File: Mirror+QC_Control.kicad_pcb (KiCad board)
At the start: 2 copper layers, 48.5 x 84 mm, 29 parts, among them J1 3220-10-0300-00, J2 Screw_Terminal_01x04, J3 Screw_Terminal_01x06, U1 LT1012, U10 LT1012, U11 LT1012, U2 LM4040DBZ-2.0, U3 LT1012, U4 LM4040DBZ-2.0, U5 LT1012, U6 LT1012, U7 Teensy4.0

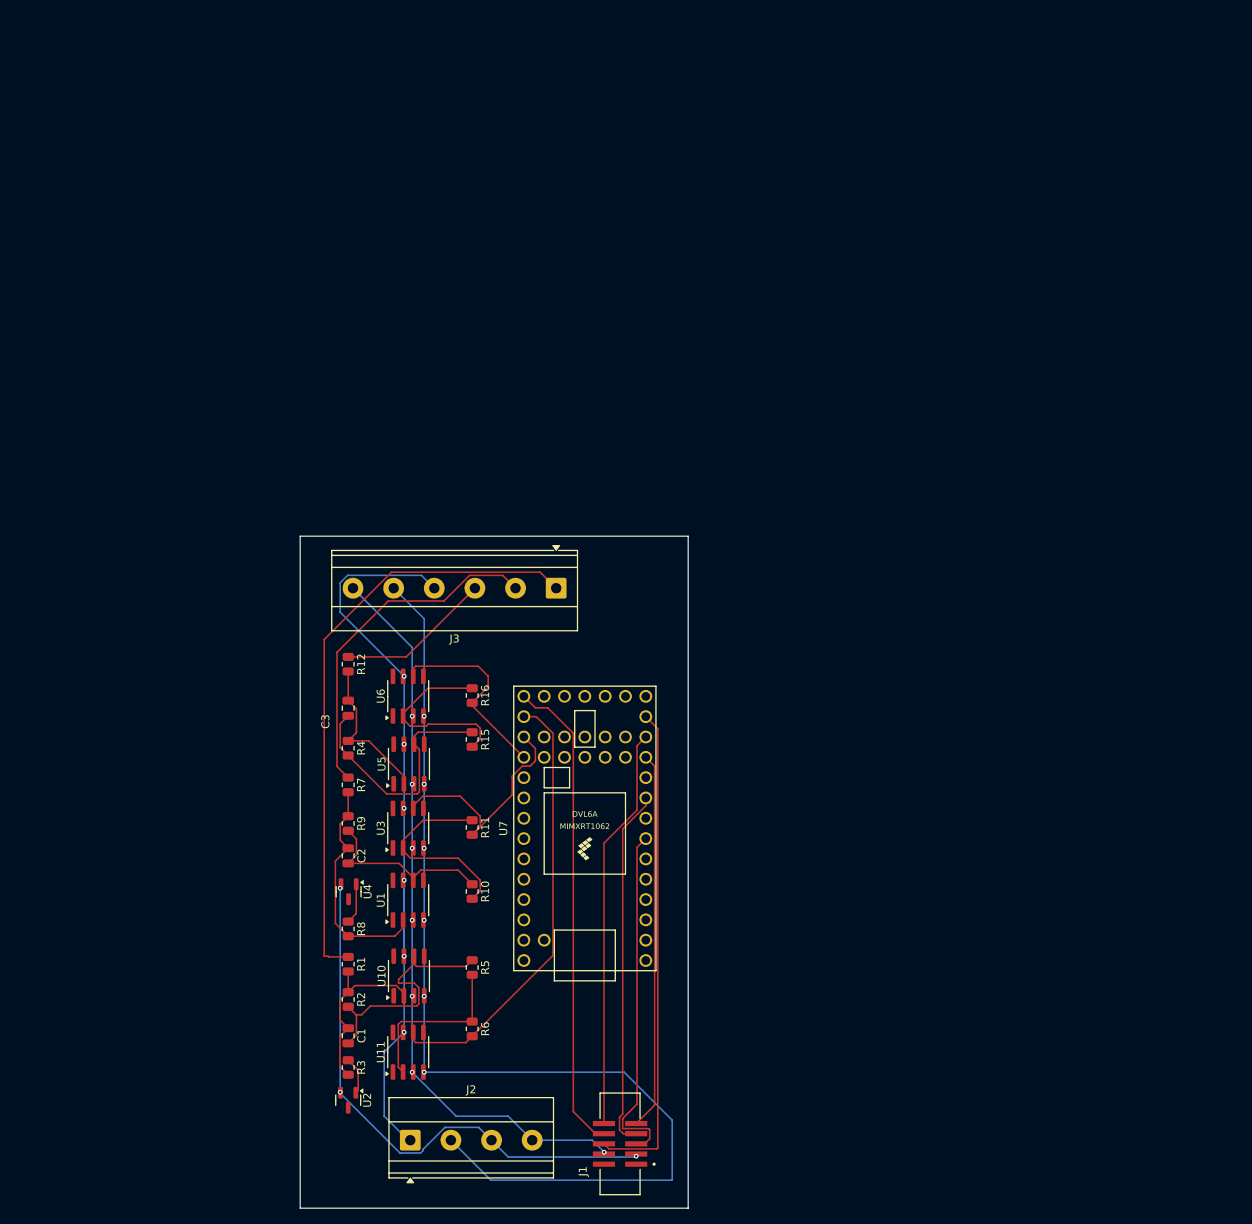
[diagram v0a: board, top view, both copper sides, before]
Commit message: changes after DR1
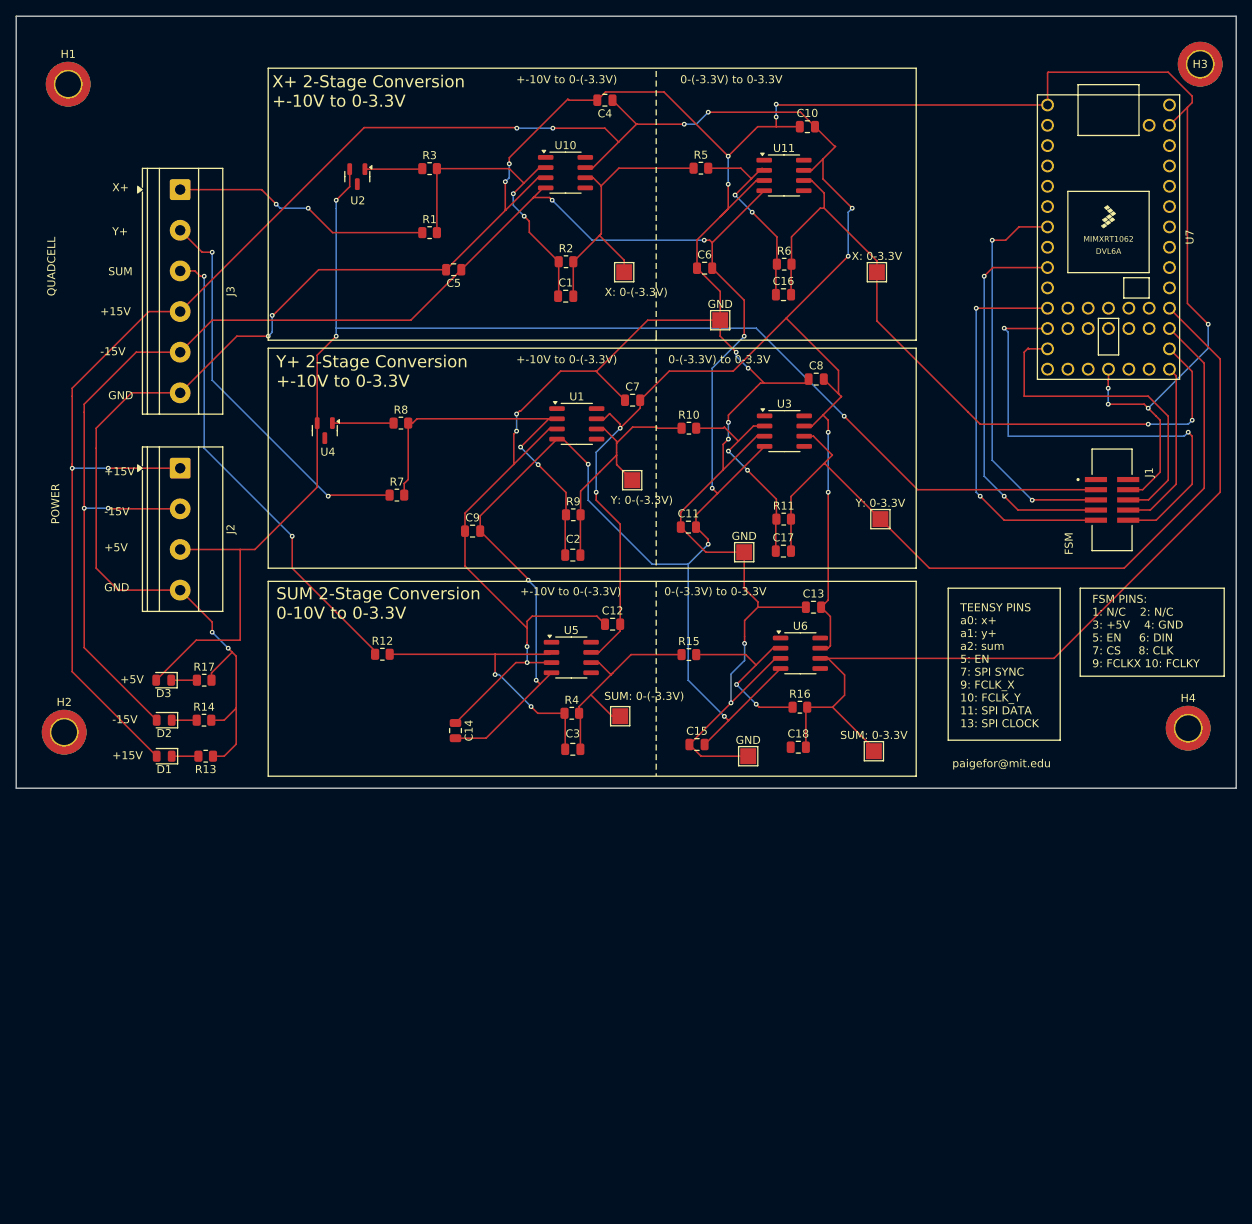
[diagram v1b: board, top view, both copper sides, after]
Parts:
- added C10: 0.1muF, Capacitor_SMD:C_0805_2012Metric, F.Cu at (118.4, 38.3)
- added C11: 0.1muF, Capacitor_SMD:C_0805_2012Metric, F.Cu at (103.5, 88.4)
- added C12: 0.1muF, Capacitor_SMD:C_0805_2012Metric, F.Cu at (94.0, 100.5)
- added C13: 0.1muF, Capacitor_SMD:C_0805_2012Metric, F.Cu at (119.2, 98.4)
- added C14: 0.1muF, Capacitor_SMD:C_0805_2012Metric, F.Cu at (74.4, 113.8)
- added C15: 0.1muF, Capacitor_SMD:C_0805_2012Metric, F.Cu at (104.6, 115.5)
- added C16: C, Capacitor_SMD:C_0805_2012Metric, F.Cu at (115.4, 59.3)
- added C17: C, Capacitor_SMD:C_0805_2012Metric, F.Cu at (115.4, 91.4)
- added C18: C, Capacitor_SMD:C_0805_2012Metric, F.Cu at (117.3, 115.9)
- added C4: 0.1muF, Capacitor_SMD:C_0805_2012Metric, F.Cu at (93.1, 35.0)
- added C5: 0.1muF, Capacitor_SMD:C_0805_2012Metric, F.Cu at (74.2, 56.2)
- added C6: 0.1muF, Capacitor_SMD:C_0805_2012Metric, F.Cu at (105.5, 56.0)
- added C7: 0.1muF, Capacitor_SMD:C_0805_2012Metric, F.Cu at (96.5, 72.5)
- added C8: 0.1muF, Capacitor_SMD:C_0805_2012Metric, F.Cu at (119.5, 69.9)
- added C9: 0.1muF, Capacitor_SMD:C_0805_2012Metric, F.Cu at (76.5, 88.9)
- added D1: 5962-XL-2012UGCTR-ND, LED_SMD:LED_0805_2012Metric, F.Cu at (38.0, 117.0)
- added D2: 5962-XL-2012UGCTR-ND, LED_SMD:LED_0805_2012Metric, F.Cu at (38.0, 112.5)
- added D3: 5962-XL-2012UGCTR-ND, LED_SMD:LED_0805_2012Metric, F.Cu at (37.9, 107.5)
- added GND: TestPoint, TestPoint:TestPoint_Pad_2.0x2.0mm, F.Cu at (111.0, 117.0)
- added GND: TestPoint, TestPoint:TestPoint_Pad_2.0x2.0mm, F.Cu at (107.5, 62.5)
- added GND: TestPoint, TestPoint:TestPoint_Pad_2.0x2.0mm, F.Cu at (110.5, 91.5)
- added H1: MountingHole_Pad_MP, MountingHole:MountingHole_3.2mm_M3_DIN965_Pad_TopBottom, F.Cu at (26.0, 33.0)
- added H2: MountingHole_Pad_MP, MountingHole:MountingHole_3.2mm_M3_DIN965_Pad_TopBottom, F.Cu at (25.5, 114.0)
- added H3: MountingHole_Pad_MP, MountingHole:MountingHole_3.2mm_M3_DIN965_Pad_TopBottom, F.Cu at (167.5, 30.5)
- added H4: MountingHole_Pad_MP, MountingHole:MountingHole_3.2mm_M3_DIN965_Pad_TopBottom, F.Cu at (166.0, 113.5)
- added R13: 1300, Resistor_SMD:R_0805_2012Metric, F.Cu at (43.2, 117.0)
- added R14: 1300, Resistor_SMD:R_0805_2012Metric, F.Cu at (43.0, 112.5)
- added R17: 300, Resistor_SMD:R_0805_2012Metric, F.Cu at (43.0, 107.5)
- added SUM: 0-(-3.3V): TestPoint, TestPoint:TestPoint_Pad_2.0x2.0mm, F.Cu at (95.0, 112.0)
- added SUM: 0-3.3V: TestPoint, TestPoint:TestPoint_Pad_2.0x2.0mm, F.Cu at (126.7, 116.4)
- added X: 0-(-3.3V): TestPoint, TestPoint:TestPoint_Pad_2.0x2.0mm, F.Cu at (95.5, 56.5)
- added X: 0-3.3V: TestPoint, TestPoint:TestPoint_Pad_2.0x2.0mm, F.Cu at (127.1, 56.5)
- added Y: 0-(-3.3V): TestPoint, TestPoint:TestPoint_Pad_2.0x2.0mm, F.Cu at (96.5, 82.5)
- added Y: 0-3.3V: TestPoint, TestPoint:TestPoint_Pad_2.0x2.0mm, F.Cu at (127.5, 87.4)
- J1: value 3220-10-0300-00 -> FSM
- moved U11 119.2 mm to (115.5, 44.4), turned to 0 degrees
- moved U2 115.5 mm to (62.1, 44.6)
- moved R3 112.8 mm to (71.2, 43.6), turned to 0 degrees
- moved R5 103.9 mm to (105.1, 43.5), turned to 0 degrees
- moved R6 103.2 mm to (115.5, 55.5), turned to 0 degrees
- moved U10 102.3 mm to (88.2, 44.1), turned to 0 degrees
- moved J1 101.3 mm to (156.5, 85.0), turned to -90 degrees
- moved U7 98.7 mm to (156.0, 52.1), turned to -90 degrees
- moved C1 96.4 mm to (88.2, 59.5), turned to 0 degrees
- moved R2 96.2 mm to (88.2, 55.2), turned to 0 degrees
- moved R1 92.0 mm to (71.2, 51.6), turned to 0 degrees
- moved J2 88.8 mm to (40.0, 81.0), turned to -90 degrees
- moved J3 68.5 mm to (40.0, 46.2), turned to -90 degrees
- moved U3 68.4 mm to (115.5, 76.4), turned to 0 degrees
- moved R10 63.9 mm to (103.6, 76.0), turned to 0 degrees
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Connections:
- net Net-(C1-Pad2) renamed /x_stage1
- net Net-(C2-Pad2) renamed /y_stage1
- net Net-(C3-Pad2) renamed /sum_stage1
- net Net-(U7-14_A0_TX3_SPDIF_OUT) renamed /x_stage2
- net Net-(U7-15_A1_RX3_SPDIF_IN) renamed /y_stage2
- net Net-(U7-16_A2_RX4_SCL1) renamed /sum_stage2
- U7 pad 1: unconnected-(U7-GND-Pad1) -> GND
- U7 pad 17: unconnected-(U7-GND-Pad17) -> GND
- U7 pad 33: +5V -> unconnected-(U7-VIN-Pad33)
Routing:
- net GND: track 91.7 -> 557.3 mm, vias 7 -> 24
- net +15V: track 97.8 -> 333.9 mm, vias 6 -> 12
- net -15V: track 132.8 -> 326.6 mm, vias 6 -> 11
- net +5V: track 68.7 -> 189.0 mm
- net /sum_stage2: track 24.6 -> 108.7 mm
- net /y_stage2: track 29.7 -> 97.7 mm
- net /x+: track 75.9 -> 32.5 mm, vias 0 -> 2
- net /sum: track 19.4 -> 59.5 mm, vias 0 -> 2
- net /SCLK: track 60.3 -> 22.1 mm
- net /x_stage2: track 55.3 -> 89.8 mm, vias 0 -> 2
- net Net-(U1--): track 28.4 -> 49.9 mm, vias 0 -> 2
- net /DIN: track 61.6 -> 41.7 mm
- net Net-(U5--): track 19.3 -> 38.1 mm, vias 0 -> 2
- net Net-(U10--): track 22.6 -> 40.9 mm, vias 0 -> 2
- net /y_stage1: track 22.6 -> 32.3 mm
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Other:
- board size 48.5 x 84 mm -> 152.5 x 96.5 mm
- board text added: "+-10V to 0-(-3.3V)"
- board text added: "+15V"
- board text added: "+5V"
- board text added: "-15V"
- board text added: "0-(-3.3V) to 0-3.3V"
- board text added: "FSM PINS: 1: N/C 2: N/C 3: +5V 4: GND 5: EN 6: DIN 7: CS 8: CLK 9: FCLKX 10: FCLKY"
- board text added: "GND"
- board text added: "POWER"
- board text added: "QUADCELL"
- board text added: "SUM"
- board text added: "SUM 2-Stage Conversion 0-10V to 0-3.3V"
- board text added: "TEENSY PINS a0: x+ a1: y+ a2: sum 5: EN 7: SPI SYNC 9: FCLK_X 10: FCLK_Y 11: SPI DATA 13: SPI CLOCK"
- board text added: "X+"
- board text added: "X+ 2-Stage Conversion +-10V to 0-3.3V"
- board text added: "Y+"
- board text added: "Y+ 2-Stage Conversion +-10V to 0-3.3V"
- board text added: "paigefor@mit.edu"

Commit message: changes since DR2
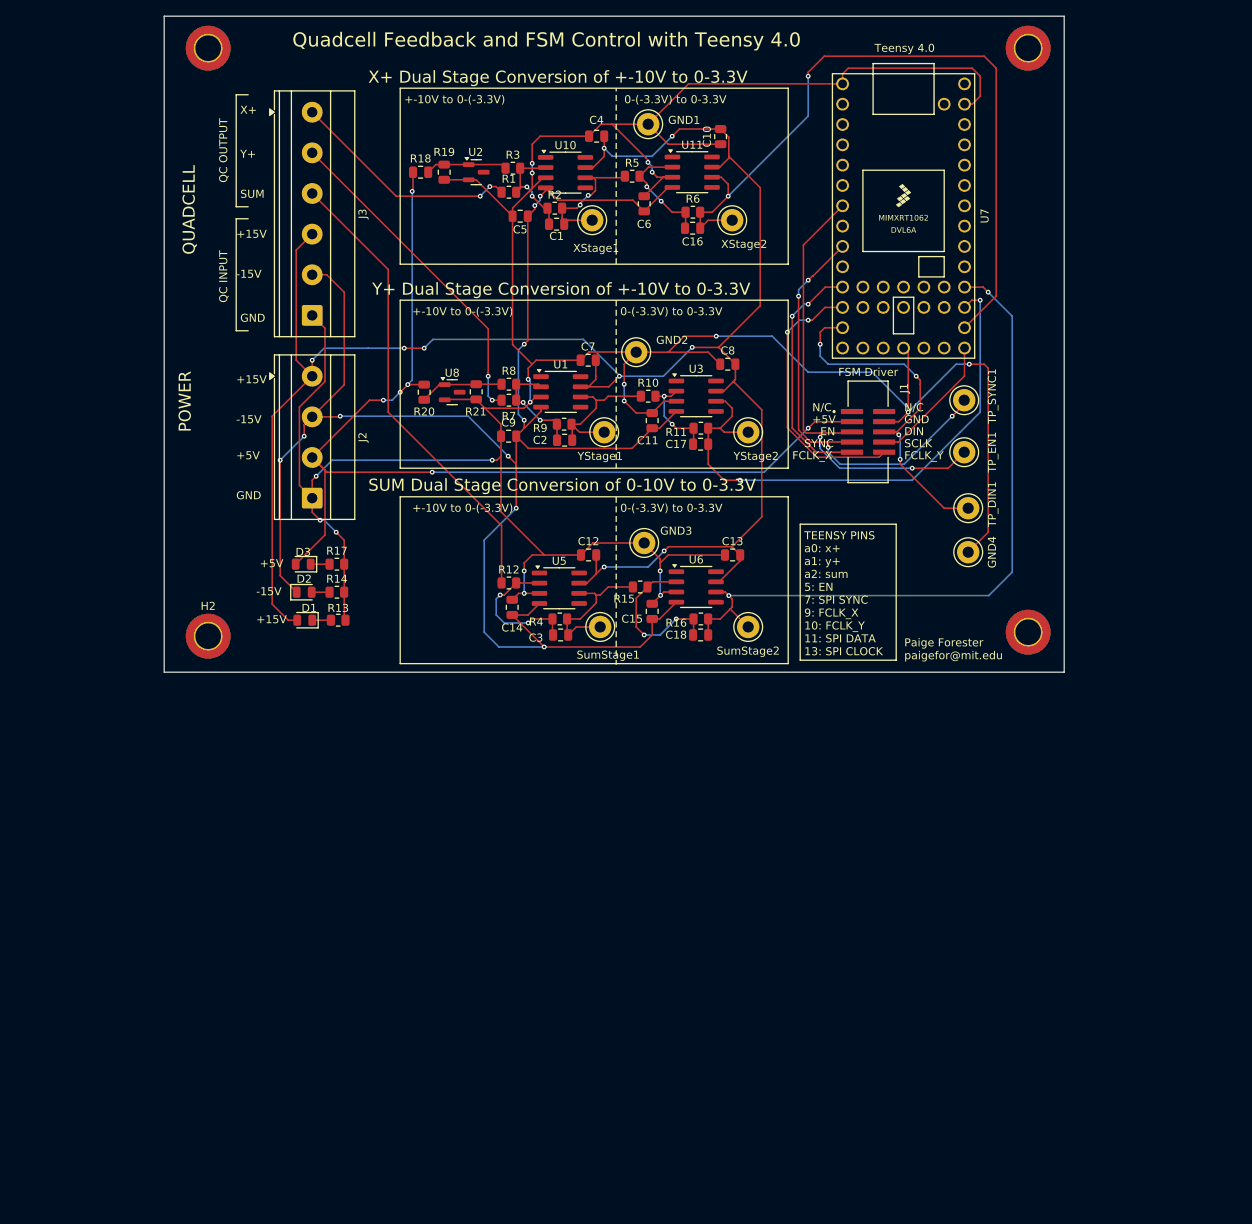
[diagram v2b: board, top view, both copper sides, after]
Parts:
- removed U4: LM4040DBZ-2.0, Package_TO_SOT_SMD:SOT-23
- added GND4: TP_GND4, TestPoint:TestPoint_Loop_D3.50mm_Drill1.4mm_Beaded, F.Cu at (138.5, 91.5)
- added R18: 750, Capacitor_SMD:C_0805_2012Metric, F.Cu at (70.0, 44.0)
- added R19: 10k, Capacitor_SMD:C_0805_2012Metric, F.Cu at (73.0, 44.0)
- added R20: 750, Capacitor_SMD:C_0805_2012Metric, F.Cu at (70.5, 71.5)
- added R21: 10k, Capacitor_SMD:C_0805_2012Metric, F.Cu at (77.0, 71.5)
- added TP_DIN1: TP_DIN, TestPoint:TestPoint_Loop_D3.50mm_Drill1.4mm_Beaded, F.Cu at (138.5, 86.0)
- added TP_EN1: TP_EN, TestPoint:TestPoint_Loop_D3.50mm_Drill1.4mm_Beaded, F.Cu at (138.0, 79.0)
- added TP_SYNC1: TP_SYNC, TestPoint:TestPoint_Loop_D3.50mm_Drill1.4mm_Beaded, F.Cu at (138.0, 72.5)
- added U8: LM4040DBZ-2.0, Package_TO_SOT_SMD:SOT-23, F.Cu at (74.0, 71.5)
- C10, C11, C12, C13, C14, C15, C4, C5, C6, C7, C8, C9: value 0.1muF -> 0.1uF
- GND1: renamed from GND; value TestPoint -> TP_GND1; footprint TestPoint:TestPoint_Pad_2.0x2.0mm -> TestPoint:TestPoint_Loop_D3.50mm_Drill1.4mm_Beaded
- GND2: renamed from GND; value TestPoint -> TP_GND2; footprint TestPoint:TestPoint_Pad_2.0x2.0mm -> TestPoint:TestPoint_Loop_D3.50mm_Drill1.4mm_Beaded
- GND3: renamed from GND; value TestPoint -> TP_GND3; footprint TestPoint:TestPoint_Pad_2.0x2.0mm -> TestPoint:TestPoint_Loop_D3.50mm_Drill1.4mm_Beaded
- J1: value FSM -> FSM Driver
- SumStage1: renamed from SUM: 0-(-3.3V); value TestPoint -> TP_sumstage1; footprint TestPoint:TestPoint_Pad_2.0x2.0mm -> TestPoint:TestPoint_Loop_D3.50mm_Drill1.4mm_Beaded
- SumStage2: renamed from SUM: 0-3.3V; value TestPoint -> TP_sumstage2; footprint TestPoint:TestPoint_Pad_2.0x2.0mm -> TestPoint:TestPoint_Loop_D3.50mm_Drill1.4mm_Beaded
- XStage1: renamed from X: 0-(-3.3V); value TestPoint -> TP_xstage1; footprint TestPoint:TestPoint_Pad_2.0x2.0mm -> TestPoint:TestPoint_Loop_D3.50mm_Drill1.4mm_Beaded
- XStage2: renamed from X: 0-3.3V; value TestPoint -> TP_xstage2; footprint TestPoint:TestPoint_Pad_2.0x2.0mm -> TestPoint:TestPoint_Loop_D3.50mm_Drill1.4mm_Beaded
- YStage1: renamed from Y: 0-(-3.3V); value TestPoint -> TP_ystage1; footprint TestPoint:TestPoint_Pad_2.0x2.0mm -> TestPoint:TestPoint_Loop_D3.50mm_Drill1.4mm_Beaded
- YStage2: renamed from Y: 0-3.3V; value TestPoint -> TP_ystage2; footprint TestPoint:TestPoint_Pad_2.0x2.0mm -> TestPoint:TestPoint_Loop_D3.50mm_Drill1.4mm_Beaded
- moved J1 31.7 mm to (126.0, 76.5)
- moved GND3 29.7 mm to (98.0, 90.3)
- moved GND2 28.4 mm to (97.0, 66.5)
- moved GND1 26.1 mm to (98.5, 38.0)
- moved U7 25.8 mm to (130.4, 49.5)
- moved D1 24.4 mm to (55.6, 100.0)
- moved R13 23.7 mm to (59.8, 100.0)
- moved D2 23.7 mm to (55.5, 96.5), turned to 0 degrees
- moved H4 23.3 mm to (146.0, 101.5)
- moved R14 23.1 mm to (59.6, 96.5)
- moved D3 22.7 mm to (55.4, 93.0)
- moved SumStage2 22.1 mm to (111.0, 100.8)
- moved R17 22.0 mm to (59.6, 93.0)
- moved H2 21.6 mm to (43.5, 102.0)
- moved H3 21.6 mm to (146.0, 28.5)
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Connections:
- D2 pad 1: Net-(D2-K) -> -15V
- D2 pad 2: -15V -> Net-(D2-A)
- R14 pad 1: Net-(D2-K) -> Net-(D2-A)
- U2 pad 2: +5V -> GND
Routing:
- net GND: track 557.3 -> 409.8 mm, vias 24 -> 19
- net -15V: track 326.6 -> 216.7 mm, vias 11 -> 10
- net +15V: track 333.9 -> 238.7 mm, vias 12 -> 9
- net +5V: track 189.0 -> 131.0 mm, vias 3 -> 6
- net Net-(U1--): track 49.9 -> 13.6 mm
- net /y_stage2: track 97.7 -> 69.9 mm, vias 0 -> 2
- net Net-(U10--): track 40.9 -> 14.1 mm
- net /FCLK_Y: track 58.4 -> 34.0 mm
- net /sum_stage2: track 108.7 -> 88.3 mm, vias 0 -> 2
- net Net-(U5--): track 38.1 -> 17.9 mm
- net /FCLK_X: track 48.3 -> 30.5 mm
- net /x_stage1: track 36.0 -> 18.8 mm, vias 0 -> 2
- net Net-(U3--): track 27.1 -> 11.7 mm
- net /y_stage1: track 32.3 -> 19.4 mm
- net Net-(U11--): track 25.9 -> 14.5 mm
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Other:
- board size 152.5 x 96.5 mm -> 112.5 x 82 mm
- board text added: "DIN"
- board text added: "EN"
- board text added: "FCLK_X"
- board text added: "FCLK_Y"
- board text added: "N/C"
- board text added: "Paige Forester paigefor@mit.edu"
- board text added: "QC INPUT"
- board text added: "QC OUTPUT"
- board text added: "Quadcell Feedback and FSM Control with Teensy 4.0"
- board text added: "SCLK"
- board text added: "SUM Dual Stage Conversion of 0-10V to 0-3.3V"
- board text added: "SYNC"
- board text added: "Teensy 4.0"
- board text added: "X+ Dual Stage Conversion of +-10V to 0-3.3V"
- board text added: "Y+ Dual Stage Conversion of +-10V to 0-3.3V"
- board text removed: "FSM PINS: 1: N/C 2: N/C 3: +5V 4: GND 5: EN 6: DIN 7: CS 8: CLK 9: FCLKX 10: FCLKY"
- board text removed: "SUM 2-Stage Conversion 0-10V to 0-3.3V"
- board text removed: "X+ 2-Stage Conversion +-10V to 0-3.3V"
- board text removed: "Y+ 2-Stage Conversion +-10V to 0-3.3V"
- board text removed: "paigefor@mit.edu"
